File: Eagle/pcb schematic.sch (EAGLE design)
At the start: 21 parts

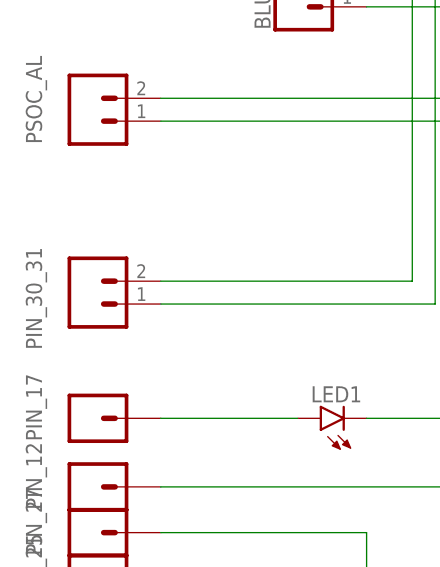
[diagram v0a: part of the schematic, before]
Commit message: case finito + modifica pcb
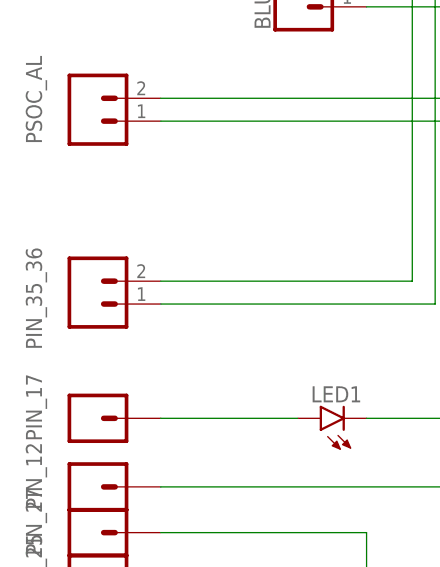
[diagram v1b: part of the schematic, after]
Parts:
- renumbered PIN_30_31 to PIN_35_36
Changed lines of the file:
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@@
 <part name="PIN_17" library="SparkFun-Connectors" deviceset="CONN_01" device=""/>
 <part name="R1" library="SparkFun-Resistors" deviceset="RESISTOR" device="AXIAL-0.3" value=" "/>
-<part name="PIN_30_31" library="SparkFun-Connectors" deviceset="CONN_02" device=""/>
+<part name="PIN_35_36" library="SparkFun-Connectors" deviceset="CONN_02" device=""/>
 <part name="BATTERY" library="SparkFun-Connectors" deviceset="CONN_02" device=""/>
 <part name="BLUETOOTH" library="SparkFun-Connectors" deviceset="CONN_04" device=""/>
@@
 <attribute name="NAME" x="-10.16" y="39.116" size="1.778" layer="95" font="vector" rot="R180" align="bottom-center"/>
 </instance>
-<instance part="PIN_30_31" gate="G$1" x="-55.88" y="53.34" smashed="yes">
+<instance part="PIN_35_36" gate="G$1" x="-55.88" y="53.34" smashed="yes">
 <attribute name="VALUE" x="-58.42" y="48.514" size="1.778" layer="96" font="vector"/>
 <attribute name="NAME" x="-61.468" y="48.26" size="1.778" layer="95" font="vector" rot="R90"/>
@@
 <wire x1="-25.4" y1="91.44" x2="-20.32" y2="91.44" width="0.1524" layer="91"/>
 <wire x1="-20.32" y1="91.44" x2="-20.32" y2="55.88" width="0.1524" layer="91"/>
-<pinref part="PIN_30_31" gate="G$1" pin="2"/>
+<pinref part="PIN_35_36" gate="G$1" pin="2"/>
 <wire x1="-20.32" y1="55.88" x2="-48.26" y2="55.88" width="0.1524" layer="91"/>
 </segment>
@@
 <wire x1="-25.4" y1="93.98" x2="-17.78" y2="93.98" width="0.1524" layer="91"/>
 <wire x1="-17.78" y1="93.98" x2="-17.78" y2="53.34" width="0.1524" layer="91"/>
-<pinref part="PIN_30_31" gate="G$1" pin="1"/>
+<pinref part="PIN_35_36" gate="G$1" pin="1"/>
 <wire x1="-17.78" y1="53.34" x2="-48.26" y2="53.34" width="0.1524" layer="91"/>
 </segment>
